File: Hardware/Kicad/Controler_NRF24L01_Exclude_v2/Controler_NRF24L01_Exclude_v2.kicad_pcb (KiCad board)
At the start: 2 copper layers, 160.2 x 60.2 mm, 82 parts, among them J1 Conn_01x02, J2 Conn_02x07_Odd_Even, J3 Conn_01x03, J4 Conn_01x03, SW1 SW_DIP_x01, SW10 SW_DIP_x01, SW11 SW_Push, SW12 SW_Push, SW13 SW_Push, SW2 SW_Push, SW3 SW_Push, SW4 SW_Push, SW5 SW_Push, SW6 SW_Push, SW7 SW_SPST, SW8 SW_Push, SW9 SW_Push, U1 STM32L412KBTx, U2 nRF24_Full, U3 MIC5219-3.3YMM, U4 PCA9685PW, U5 PCF8574TS

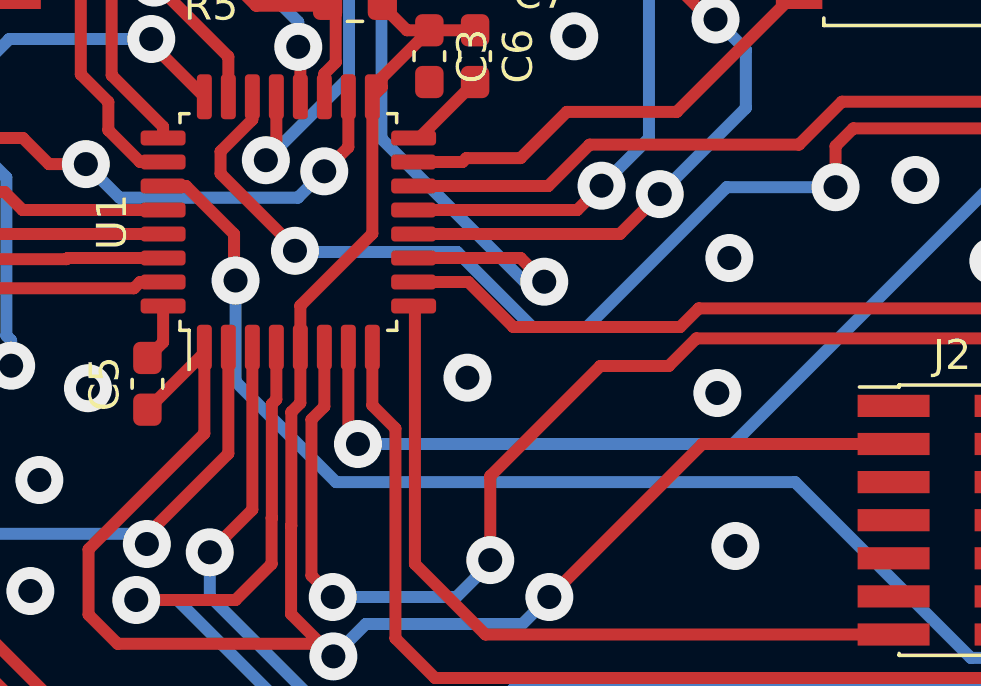
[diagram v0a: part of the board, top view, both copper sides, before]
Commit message: V.2.3
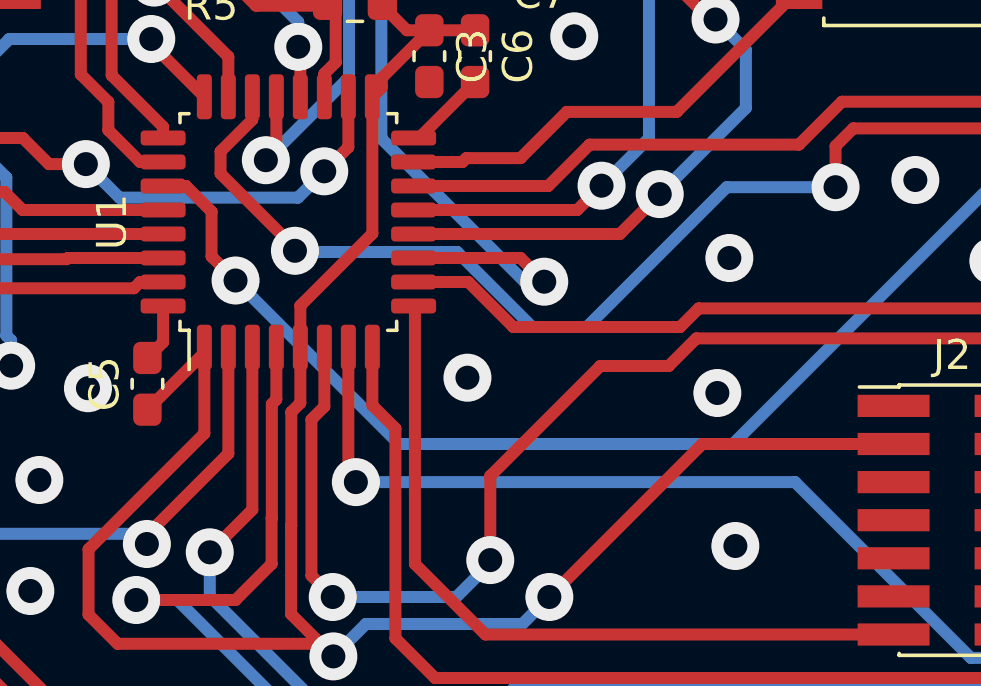
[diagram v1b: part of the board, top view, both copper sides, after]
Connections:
- U1 pad 27: POWER_CHECK -> Order_Search
- U1 pad 7: Order_Search -> POWER_CHECK
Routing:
- net POWER_CHECK: track 54.6 -> 45.8 mm
- net Order_Search: track 79.6 -> 87.2 mm
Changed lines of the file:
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@@
   (net 83 "unconnected-(U5-P6-Pad19)")
   (net 84 "unconnected-(U5-P0-Pad10)")
-  (net 85 "Net-(U3-IN)")
+  (net 85 "Net-(FLG05-pwr)")
   (footprint "Resistor_SMD:R_0603_1608Metric_Pad0.98x0.95mm_HandSolder" (layer "F.Cu")
     (at 150.368 74.422)
@@
       (net 72 "unconnected-(U3-EN-Pad1)") (pinfunction "EN") (pintype "input+no_connect"))
     (pad "2" smd roundrect (at -2.1125 -0.325) (size 1.625 0.4) (layers "F.Cu" "F.Paste" "F.Mask") (roundrect_rratio 0.25)
-      (net 85 "Net-(U3-IN)") (pinfunction "IN") (pintype "power_in"))
+      (net 85 "Net-(FLG05-pwr)") (pinfunction "IN") (pintype "power_in"))
     (pad "3" smd roundrect (at -2.1125 0.325) (size 1.625 0.4) (layers "F.Cu" "F.Paste" "F.Mask") (roundrect_rratio 0.25)
       (net 5 "Glob_Alim") (pinfunction "OUT") (pintype "power_out"))
@@
       (net 3 "Li-ion") (pintype "passive"))
     (pad "2" smd rect (at 3.81 0 90) (size 1.6 0.76) (layers "F.Cu" "F.Paste" "F.Mask")
-      (net 85 "Net-(U3-IN)") (pintype "passive"))
+      (net 85 "Net-(FLG05-pwr)") (pintype "passive"))
     (model "${KICAD6_3DMODEL_DIR}/Button_Switch_SMD.3dshapes/SW_DIP_SPSTx01_Slide_Copal_CHS-01B_W7.62mm_P1.27mm.wrl"
       (offset (xyz 0 0 0))
@@
       (net 52 "B_Button") (pinfunction "PA0") (pintype "bidirectional"))
     (pad "7" smd roundrect (at -4.175 2 90) (size 1.5 0.5) (layers "F.Cu" "F.Paste" "F.Mask") (roundrect_rratio 0.25)
-      (net 65 "Order_Search") (pinfunction "PA1") (pintype "bidirectional"))
+      (net 1 "POWER_CHECK") (pinfunction "PA1") (pintype "bidirectional"))
     (pad "8" smd roundrect (at -4.175 2.8 90) (size 1.5 0.5) (layers "F.Cu" "F.Paste" "F.Mask") (roundrect_rratio 0.25)
       (net 48 "USART2_TX") (pinfunction "PA2") (pintype "bidirectional"))
@@
       (net 62 "DIODE_OE") (pinfunction "PB3") (pintype "bidirectional"))
     (pad "27" smd roundrect (at 1.2 -4.175 90) (size 0.5 1.5) (layers "F.Cu" "F.Paste" "F.Mask") (roundrect_rratio 0.25)
-      (net 1 "POWER_CHECK") (pinfunction "PB4") (pintype "bidirectional"))
+      (net 65 "Order_Search") (pinfunction "PB4") (pintype "bidirectional"))
     (pad "28" smd roundrect (at 0.4 -4.175 90) (size 0.5 1.5) (layers "F.Cu" "F.Paste" "F.Mask") (roundrect_rratio 0.25)
       (net 49 "NES{slash}SNES_switcher") (pinfunction "PB5") (pintype "bidirectional"))
@@
   )
   (segment (start 171.4 111.425) (end 173.35 111.425) (width 0.4) (layer "F.Cu") (net 1))
-  (segment (start 133.21 100.92) (end 133.24 100.95) (width 0.4) (layer "F.Cu") (net 1))
-  (segment (start 130.825 97.8) (end 131.588173 97.8) (width 0.4) (layer "F.Cu") (net 1))
+  (segment (start 137 107.42) (end 137.25 107.67) (width 0.4) (layer "F.Cu") (net 1))
   (segment (start 173.35 111.425) (end 173.4 111.475) (width 0.4) (layer "F.Cu") (net 1))
-  (segment (start 133.19 99.401827) (end 133.19 100.92) (width 0.4) (layer "F.Cu") (net 1))
-  (segment (start 133.19 100.92) (end 133.21 100.92) (width 0.4) (layer "F.Cu") (net 1))
+  (segment (start 137 103.175) (end 137 107.42) (width 0.4) (layer "F.Cu") (net 1))
   (segment (start 169.295 113.53) (end 171.4 111.425) (width 0.4) (layer "F.Cu") (net 1))
   (segment (start 173.4 111.475) (end 173.4 109.7125) (width 0.4) (layer "F.Cu") (net 1))
   (segment (start 168.8 113.53) (end 169.295 113.53) (width 0.4) (layer "F.Cu") (net 1))
-  (segment (start 131.588173 97.8) (end 133.19 99.401827) (width 0.4) (layer "F.Cu") (net 1))
+  (via (at 137.25 107.67) (size 1.6) (drill 0.8) (layers "F.Cu" "B.Cu") (net 1))
   (via (at 168.8 113.53) (size 1.6) (drill 0.8) (layers "F.Cu" "B.Cu") (net 1))
-  (via (at 133.24 100.95) (size 1.6) (drill 0.8) (layers "F.Cu" "B.Cu") (net 1))
   (segment (start 151.89 107.67) (end 157.75 113.53) (width 0.4) (layer "B.Cu") (net 1))
+  (segment (start 137.25 107.67) (end 151.89 107.67) (width 0.4) (layer "B.Cu") (net 1))
   (segment (start 157.75 113.53) (end 168.8 113.53) (width 0.4) (layer "B.Cu") (net 1))
-  (segment (start 136.59 107.67) (end 151.89 107.67) (width 0.4) (layer "B.Cu") (net 1))
-  (segment (start 133.24 104.32) (end 136.59 107.67) (width 0.4) (layer "B.Cu") (net 1))
-  (segment (start 133.24 100.95) (end 133.24 104.32) (width 0.4) (layer "B.Cu") (net 1))
   (segment (start 137.3 86.85) (end 137.05 87.1) (width 0.4) (layer "F.Cu") (net 2))
   (segment (start 138.35 87.8) (end 138.35 86.9) (width 0.4) (layer "F.Cu") (net 2))
@@
   (segment (start 140.803639 97) (end 140.932642 96.870998) (width 0.4) (layer "F.Cu") (net 64))
   (segment (start 139.175 97) (end 140.803639 97) (width 0.4) (layer "F.Cu") (net 64))
+  (segment (start 132.44 98.651827) (end 132.44 100.15) (width 0.4) (layer "F.Cu") (net 65))
+  (segment (start 132.44 100.15) (end 133.24 100.95) (width 0.4) (layer "F.Cu") (net 65))
+  (segment (start 130.825 97.8) (end 131.588173 97.8) (width 0.4) (layer "F.Cu") (net 65))
   (segment (start 180.489613 70.764613) (end 180.489613 70.8395) (width 0.4) (layer "F.Cu") (net 65))
   (segment (start 176.475 66.75) (end 180.489613 70.764613) (width 0.4) (layer "F.Cu") (net 65))
-  (segment (start 137 103.175) (end 137 106.08) (width 0.4) (layer "F.Cu") (net 65))
-  (segment (start 137 106.08) (end 137.32 106.4) (width 0.4) (layer "F.Cu") (net 65))
+  (segment (start 131.588173 97.8) (end 132.44 98.651827) (width 0.4) (layer "F.Cu") (net 65))
   (segment (start 176.475 66.75) (end 168.525 66.75) (width 0.4) (layer "F.Cu") (net 65))
-  (via (at 137.32 106.4) (size 1.6) (drill 0.8) (layers "F.Cu" "B.Cu") (net 65))
   (via (at 180.489613 70.8395) (size 1.6) (drill 0.8) (layers "F.Cu" "B.Cu") (net 65))
-  (segment (start 137.32 106.4) (end 149.82 106.4) (width 0.4) (layer "B.Cu") (net 65))
+  (via (at 133.24 100.95) (size 1.6) (drill 0.8) (layers "F.Cu" "B.Cu") (net 65))
+  (segment (start 162.92 91.98) (end 166.55 88.35) (width 0.4) (layer "B.Cu") (net 65))
+  (segment (start 138.69 106.4) (end 149.82 106.4) (width 0.4) (layer "B.Cu") (net 65))
   (segment (start 170.8 80.529113) (end 180.489613 70.8395) (width 0.4) (layer "B.Cu") (net 65))
+  (segment (start 162.92 93.3) (end 162.92 91.98) (width 0.4) (layer "B.Cu") (net 65))
   (segment (start 149.82 106.4) (end 162.92 93.3) (width 0.4) (layer "B.Cu") (net 65))
-  (segment (start 162.92 91.98) (end 166.55 88.35) (width 0.4) (layer "B.Cu") (net 65))
-  (segment (start 166.55 88.35) (end 169.65 88.35) (width 0.4) (layer "B.Cu") (net 65))
   (segment (start 169.65 88.35) (end 170.8 87.2) (width 0.4) (layer "B.Cu") (net 65))
-  (segment (start 162.92 93.3) (end 162.92 91.98) (width 0.4) (layer "B.Cu") (net 65))
   (segment (start 170.8 87.2) (end 170.8 80.529113) (width 0.4) (layer "B.Cu") (net 65))
+  (segment (start 166.55 88.35) (end 169.65 88.35) (width 0.4) (layer "B.Cu") (net 65))
+  (segment (start 133.24 100.95) (end 138.69 106.4) (width 0.4) (layer "B.Cu") (net 65))
   (segment (start 136.7805 67.4895) (end 136.7805 79.077727) (width 0.4) (layer "F.Cu") (net 66))
   (segment (start 142.2 64.6) (end 139.67 64.6) (width 0.4) (layer "F.Cu") (net 66))

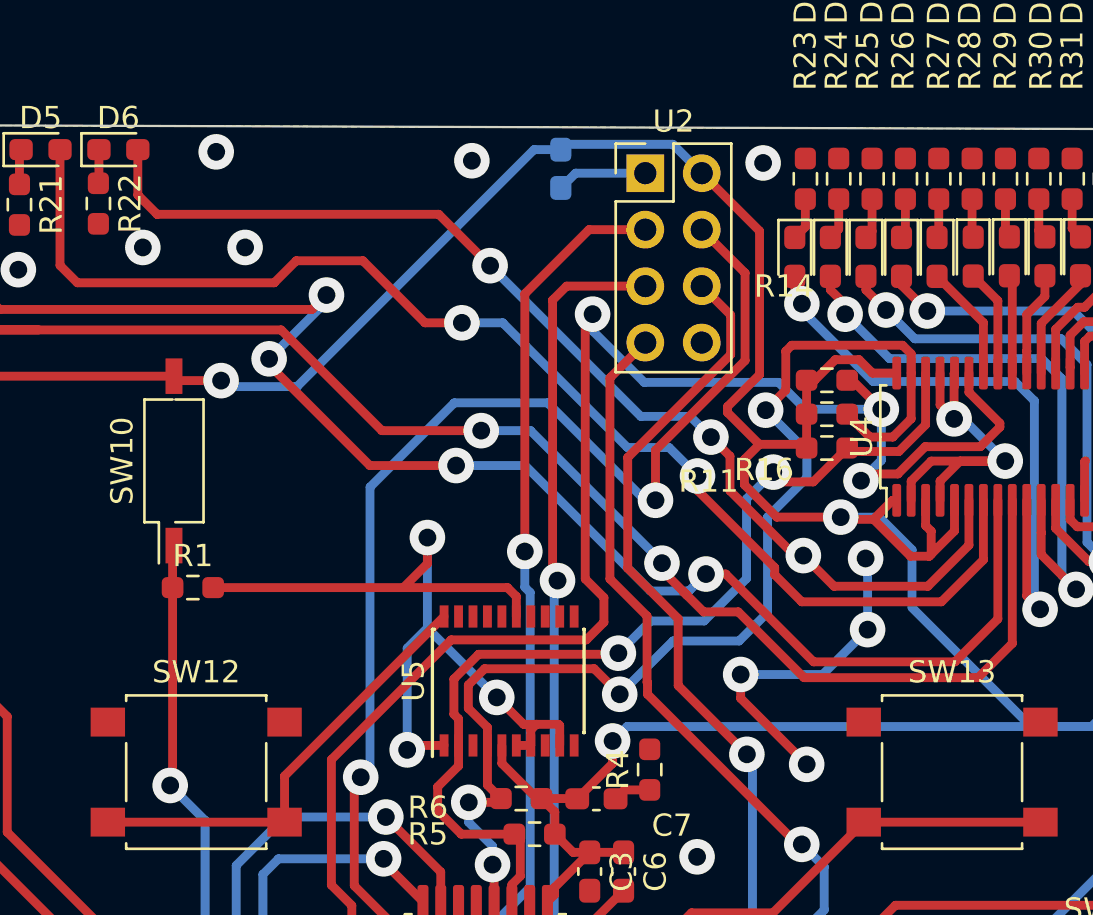
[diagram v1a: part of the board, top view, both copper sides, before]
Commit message: V.2.4
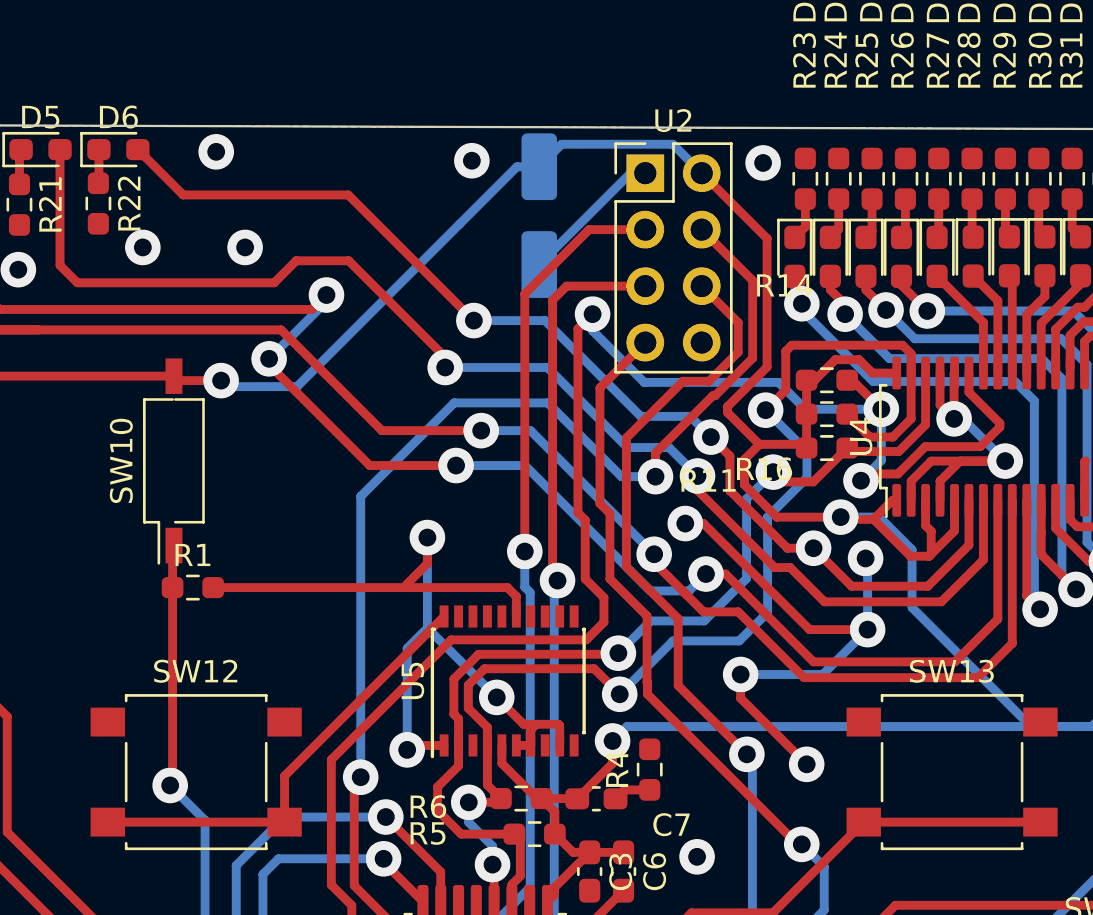
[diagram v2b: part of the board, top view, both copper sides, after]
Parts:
- C1: value 100uF -> 22uF; footprint Capacitor_SMD:C_0603_1608Metric_Pad1.08x0.95mm_HandSolder -> Capacitor_SMD:CP_Elec_5x5.4
- moved C1 2.32 mm to (137.4, 64.0)
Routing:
- net GND: track 82.2 -> 94.8 mm, vias 66 -> 67
- net Net-(D6-A): track 50.4 -> 49.2 mm
- net CSN_nRF24: track 51.9 -> 50.7 mm
- net MOSI: track 42.7 -> 43.7 mm
